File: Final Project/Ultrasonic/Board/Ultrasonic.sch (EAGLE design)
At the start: 17 parts, among them IC1 ATTINY44-SSU, IC3 OPAMPSOT23-5

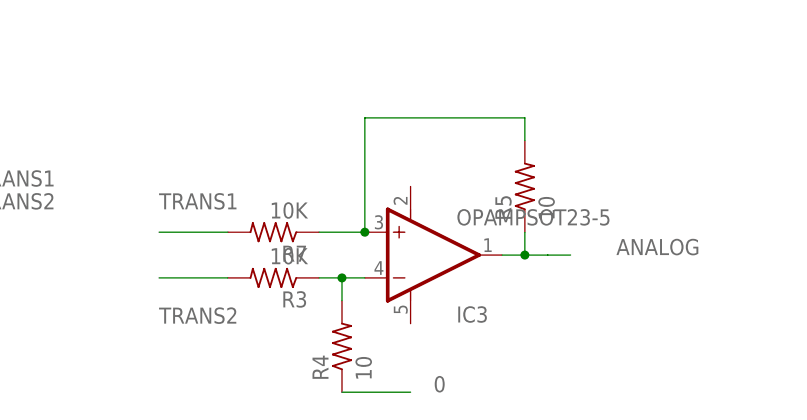
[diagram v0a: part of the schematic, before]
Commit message: Ultrasonic Fail :(
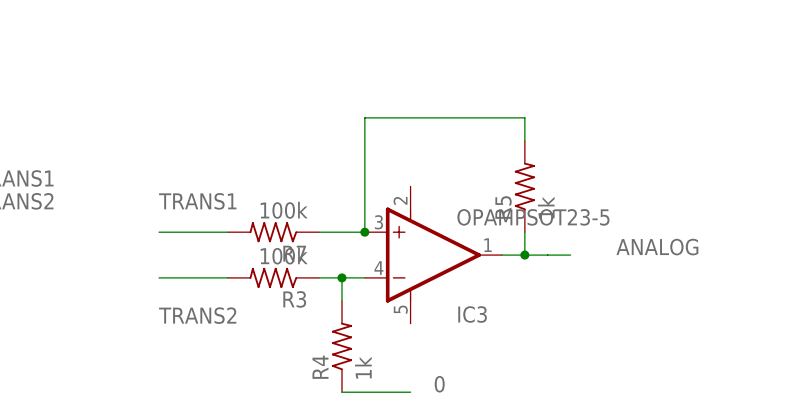
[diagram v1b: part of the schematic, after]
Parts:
- R3, R7: value 10K -> 100k
- R4, R5: value 10 -> 1k
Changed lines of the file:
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@@
 <part name="U$5" library="fab" deviceset="PINHD-2X2-SMD" device=""/>
 <part name="U$6" library="fab" deviceset="PINHD-2X2-SMD" device=""/>
-<part name="R3" library="fab" deviceset="RES-US" device="1206FAB" value="10K"/>
-<part name="R4" library="fab" deviceset="RES-US" device="1206FAB" value="10"/>
-<part name="R5" library="fab" deviceset="RES-US" device="1206FAB" value="10"/>
-<part name="R7" library="fab" deviceset="RES-US" device="1206FAB" value="10K"/>
+<part name="R3" library="fab" deviceset="RES-US" device="1206FAB" value="100k"/>
+<part name="R4" library="fab" deviceset="RES-US" device="1206FAB" value="1k"/>
+<part name="R5" library="fab" deviceset="RES-US" device="1206FAB" value="1k"/>
+<part name="R7" library="fab" deviceset="RES-US" device="1206FAB" value="100k"/>
 <part name="R6" library="fab" deviceset="RES-US" device="1206FAB" value="10"/>
 <part name="R8" library="fab" deviceset="RES-US" device="1206FAB" value="10"/>
